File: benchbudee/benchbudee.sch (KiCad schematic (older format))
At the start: 0 parts

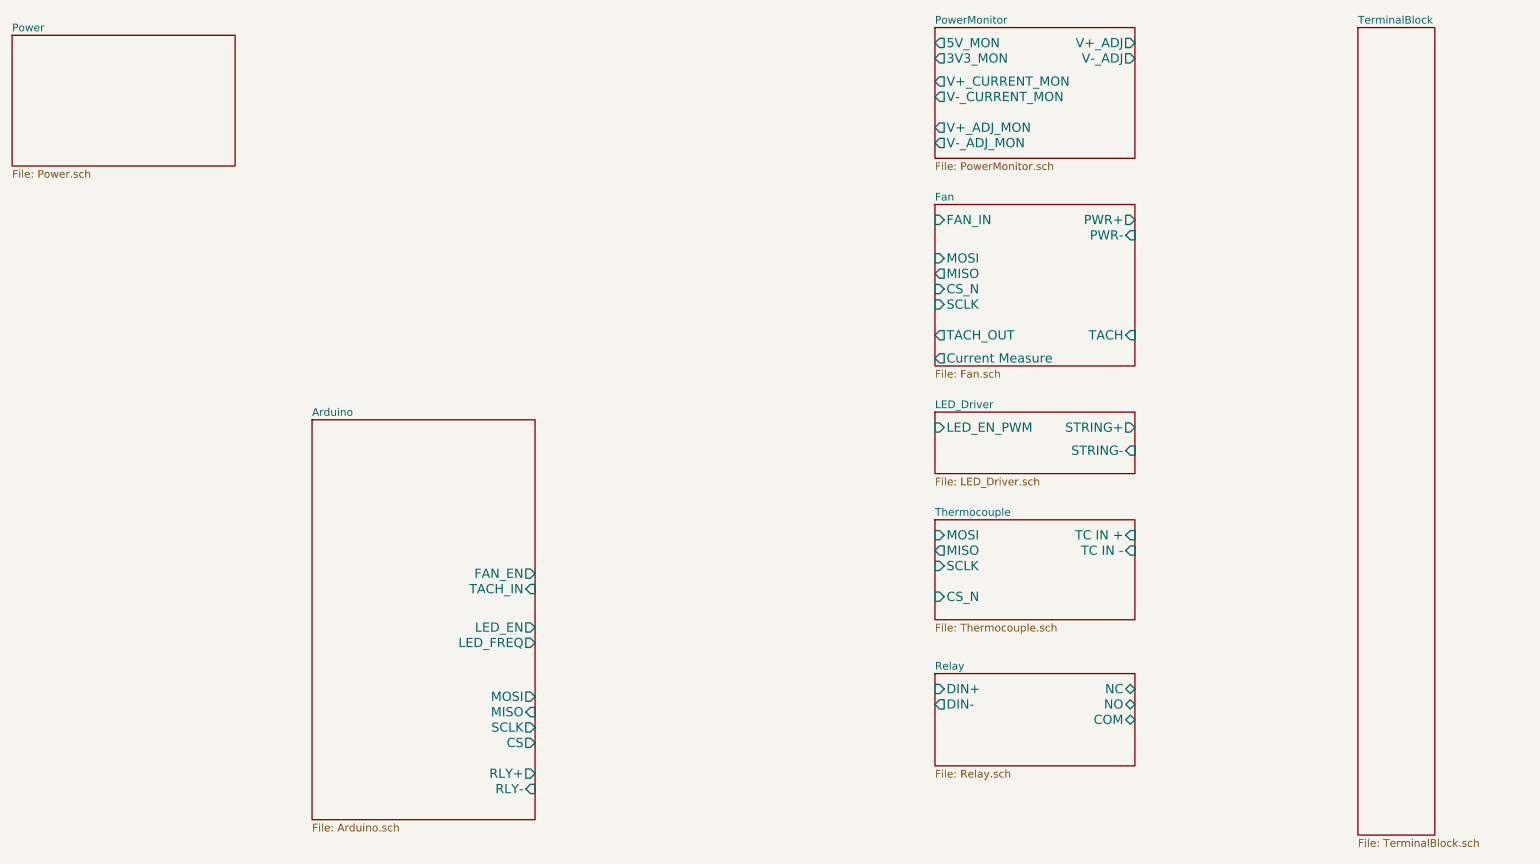
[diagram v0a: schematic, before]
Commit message: Setting up for layout
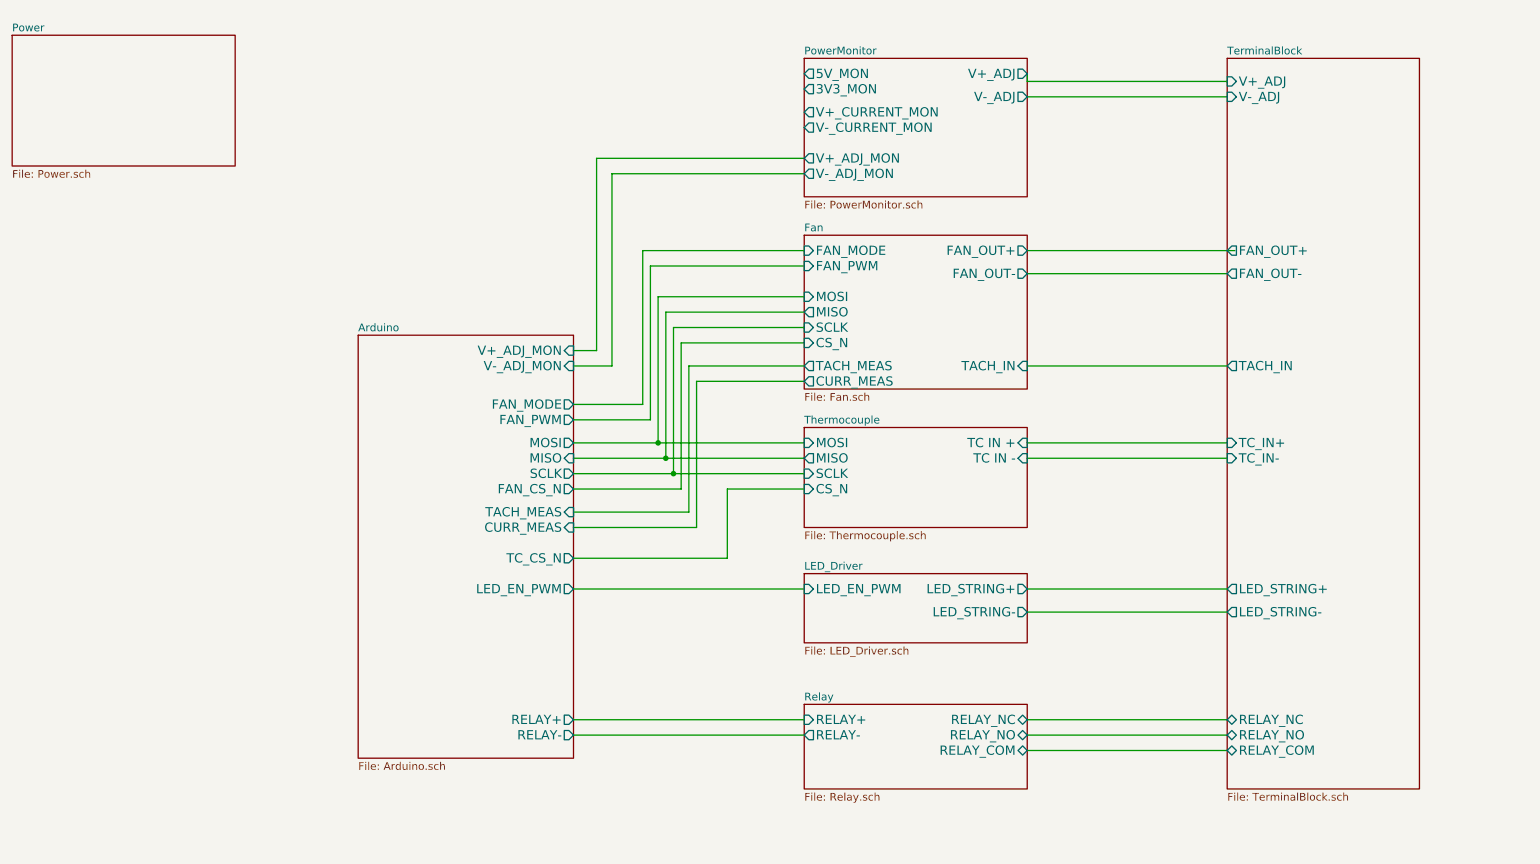
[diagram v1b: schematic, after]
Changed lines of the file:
@@
 LIBS:benchbudee-custom
 LIBS:benchbudee-cache
-EELAYER 27 0
+EELAYER 24 0
 EELAYER END
 $Descr A4 11693 8268
@@
 $EndDescr
 $Sheet
-S 3050 3450 1450 2600
-U 52F13E2E
-F0 "Arduino" 50
-F1 "Arduino.sch" 50
-F2 "RLY+" O R 4500 5750 60
-F3 "RLY-" I R 4500 5850 60
-F4 "MOSI" O R 4500 5250 60
-F5 "MISO" I R 4500 5350 60
-F6 "SCLK" O R 4500 5450 60
-F7 "CS" O R 4500 5550 60
-F8 "LED_EN" O R 4500 4800 60
-F9 "LED_FREQ" O R 4500 4900 60
-F10 "FAN_EN" O R 4500 4450 60
-F11 "TACH_IN" I R 4500 4550 60
-$EndSheet
-$Sheet
-S 7100 4100 1300 650
+S 6250 3500 1450 650
 U 52F13E8B
 F0 "Thermocouple" 50
 F1 "Thermocouple.sch" 50
-F2 "TC IN +" I R 8400 4200 60
-F3 "TC IN -" I R 8400 4300 60
-F4 "MOSI" I L 7100 4200 60
-F5 "MISO" O L 7100 4300 60
-F6 "SCLK" I L 7100 4400 60
-F7 "CS_N" I L 7100 4600 60
-$EndSheet
-$Sheet
-S 7100 5100 1300 600
+F2 "TC IN +" I R 7700 3600 60
+F3 "TC IN -" I R 7700 3700 60
+F4 "MOSI" I L 6250 3600 60
+F5 "MISO" O L 6250 3700 60
+F6 "SCLK" I L 6250 3800 60
+F7 "CS_N" I L 6250 3900 60
+$EndSheet
+$Sheet
+S 6250 5300 1450 550
 U 52F13E9E
 F0 "Relay" 50
 F1 "Relay.sch" 50
-F2 "DIN+" I L 7100 5200 60
-F3 "DIN-" O L 7100 5300 60
-F4 "NC" B R 8400 5200 60
-F5 "NO" B R 8400 5300 60
-F6 "COM" B R 8400 5400 60
+F2 "RELAY_NC" B R 7700 5400 60
+F3 "RELAY_NO" B R 7700 5500 60
+F4 "RELAY_COM" B R 7700 5600 60
+F5 "RELAY+" I L 6250 5400 60
+F6 "RELAY-" O L 6250 5500 60
 $EndSheet
 $Sheet
@@
 $EndSheet
 $Sheet
-S 7100 3400 1300 400
+S 6250 4450 1450 450
 U 52F1408A
 F0 "LED_Driver" 50
 F1 "LED_Driver.sch" 50
-F2 "STRING+" O R 8400 3500 60
-F3 "STRING-" I R 8400 3650 60
-F4 "LED_EN_PWM" I L 7100 3500 60
-$EndSheet
-$Sheet
-S 9850 900  500  5250
+F2 "LED_EN_PWM" I L 6250 4550 60
+F3 "LED_STRING+" O R 7700 4550 60
+F4 "LED_STRING-" O R 7700 4700 60
+$EndSheet
+$Sheet
+S 6250 1100 1450 900
+U 52FC1BE1
+F0 "PowerMonitor" 50
+F1 "PowerMonitor.sch" 50
+F2 "V+_ADJ" O R 7700 1200 60
+F3 "V-_ADJ" O R 7700 1350 60
+F4 "3V3_MON" O L 6250 1300 60
+F5 "5V_MON" O L 6250 1200 60
+F6 "V+_ADJ_MON" O L 6250 1750 60
+F7 "V-_ADJ_MON" O L 6250 1850 60
+F8 "V+_CURRENT_MON" O L 6250 1450 60
+F9 "V-_CURRENT_MON" O L 6250 1550 60
+$EndSheet
+Wire Wire Line
+	7700 1200 7700 1250
+Wire Wire Line
+	7700 1250 9000 1250
+Wire Wire Line
+	7700 1350 9000 1350
+Wire Wire Line
+	7700 2350 9050 2350
+Wire Wire Line
+	7700 2500 9000 2500
+Wire Wire Line
+	7700 3100 9000 3100
+Wire Wire Line
+	7700 5400 9000 5400
+Wire Wire Line
+	7700 5500 9000 5500
+Wire Wire Line
+	7700 5600 9000 5600
+Wire Wire Line
+	4750 3000 4900 3000
+Wire Wire Line
+	4900 3000 4900 1750
+Wire Wire Line
+	4900 1750 6250 1750
+Wire Wire Line
+	4750 3100 5000 3100
+Wire Wire Line
+	5000 3100 5000 1850
+Wire Wire Line
+	5000 1850 6250 1850
+Wire Wire Line
+	4750 3450 5250 3450
+Wire Wire Line
+	5250 3450 5250 2450
+Wire Wire Line
+	5250 2450 6250 2450
+Wire Wire Line
+	4750 3600 5300 3600
+Wire Wire Line
+	5300 3600 6250 3600
+Wire Wire Line
+	5300 3600 5300 2650
+Wire Wire Line
+	5300 2650 6250 2650
+Wire Wire Line
+	4750 3700 5350 3700
+Wire Wire Line
+	5350 3700 6250 3700
+Wire Wire Line
+	5350 3700 5350 2750
+Wire Wire Line
+	5350 2750 6250 2750
+Wire Wire Line
+	5400 3800 5400 2850
+Wire Wire Line
+	5400 2850 6250 2850
+Wire Wire Line
+	4750 4050 5500 4050
+Wire Wire Line
+	5500 4050 5500 3100
+Wire Wire Line
+	5500 3100 6250 3100
+Wire Wire Line
+	4750 4150 5550 4150
+Wire Wire Line
+	5550 4150 5550 3200
+Wire Wire Line
+	5550 3200 6250 3200
+Wire Wire Line
+	4750 4550 6250 4550
+$Sheet
+S 9000 1100 1250 4750
 U 52F140D2
 F0 "TerminalBlock" 50
 F1 "TerminalBlock.sch" 50
-$EndSheet
-$Sheet
-S 7100 2050 1300 1050
+F2 "V+_ADJ" I L 9000 1250 60
+F3 "V-_ADJ" I L 9000 1350 60
+F4 "FAN_OUT+" O L 9000 2350 60
+F5 "FAN_OUT-" O L 9000 2500 60
+F6 "TACH_IN" O L 9000 3100 60
+F7 "LED_STRING+" O L 9000 4550 60
+F8 "LED_STRING-" O L 9000 4700 60
+F9 "TC_IN+" I L 9000 3600 60
+F10 "TC_IN-" I L 9000 3700 60
+F11 "RELAY_NO" B L 9000 5500 60
+F12 "RELAY_NC" B L 9000 5400 60
+F13 "RELAY_COM" B L 9000 5600 60
+$EndSheet
+Wire Wire Line
+	7700 3600 9000 3600
+Wire Wire Line
+	7700 3700 9000 3700
+Wire Wire Line
+	7700 4550 9000 4550
+Wire Wire Line
+	7700 4700 9000 4700
+Connection ~ 5300 3600
+Connection ~ 5350 3700
+Wire Wire Line
+	4750 3800 5400 3800
+Wire Wire Line
+	5400 3800 6250 3800
+Connection ~ 5400 3800
+Wire Wire Line
+	4750 3900 5450 3900
+Wire Wire Line
+	5450 3900 5450 2950
+Wire Wire Line
+	5450 2950 6250 2950
+Wire Wire Line
+	4750 4350 5750 4350
+Wire Wire Line
+	5750 4350 5750 3900
+Wire Wire Line
+	5750 3900 6250 3900
+Wire Wire Line
+	4750 5400 6250 5400
+Wire Wire Line
+	6250 5500 4750 5500
+Wire Wire Line
+	4750 3350 5200 3350
+Wire Wire Line
+	5200 3350 5200 2350
+Wire Wire Line
+	5200 2350 6250 2350
+$Sheet
+S 6250 2250 1450 1000
 U 52F140AA
 F0 "Fan" 50
 F1 "Fan.sch" 50
-F2 "PWR+" O R 8400 2150 60
-F3 "PWR-" I R 8400 2250 60
-F4 "TACH" I R 8400 2900 60
-F5 "TACH_OUT" O L 7100 2900 60
-F6 "FAN_IN" I L 7100 2150 60
-F7 "Current Measure" O L 7100 3050 60
-F8 "MOSI" I L 7100 2400 60
-F9 "MISO" O L 7100 2500 60
-F10 "CS_N" I L 7100 2600 60
-F11 "SCLK" I L 7100 2700 60
-$EndSheet
-$Sheet
-S 7100 900  1300 850
-U 52FC1BE1
-F0 "PowerMonitor" 50
-F1 "PowerMonitor.sch" 50
-F2 "V+_ADJ" O R 8400 1000 60
-F3 "V-_ADJ" O R 8400 1100 60
-F4 "3V3_MON" O L 7100 1100 60
-F5 "5V_MON" O L 7100 1000 60
-F6 "V+_ADJ_MON" O L 7100 1550 60
-F7 "V-_ADJ_MON" O L 7100 1650 60
-F8 "V+_CURRENT_MON" O L 7100 1250 60
-F9 "V-_CURRENT_MON" O L 7100 1350 60
+F2 "MOSI" I L 6250 2650 60
+F3 "MISO" O L 6250 2750 60
+F4 "CS_N" I L 6250 2950 60
+F5 "SCLK" I L 6250 2850 60
+F6 "FAN_OUT+" O R 7700 2350 60
+F7 "FAN_OUT-" O R 7700 2500 60
+F8 "TACH_IN" I R 7700 3100 60
+F9 "TACH_MEAS" O L 6250 3100 60
+F10 "CURR_MEAS" O L 6250 3200 60
+F11 "FAN_PWM" I L 6250 2450 60
+F12 "FAN_MODE" I L 6250 2350 60
+$EndSheet
+$Sheet
+S 3350 2900 1400 2750
+U 52F13E2E
+F0 "Arduino" 50
+F1 "Arduino.sch" 50
+F2 "MOSI" O R 4750 3600 60
+F3 "MISO" I R 4750 3700 60
+F4 "SCLK" O R 4750 3800 60
+F5 "RELAY-" O R 4750 5500 60
+F6 "RELAY+" O R 4750 5400 60
+F7 "TACH_MEAS" I R 4750 4050 60
+F8 "CURR_MEAS" I R 4750 4150 60
+F9 "V+_ADJ_MON" I R 4750 3000 60
+F10 "V-_ADJ_MON" I R 4750 3100 60
+F11 "LED_EN_PWM" O R 4750 4550 60
+F12 "FAN_CS_N" O R 4750 3900 60
+F13 "TC_CS_N" O R 4750 4350 60
+F14 "FAN_PWM" O R 4750 3450 60
+F15 "FAN_MODE" O R 4750 3350 60
 $EndSheet
 $EndSCHEMATC

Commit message: Relay module footprints done
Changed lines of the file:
@@
 	5250 2450 6250 2450
 Wire Wire Line
-	4750 3600 5300 3600
-Wire Wire Line
-	5300 3600 6250 3600
+	4750 3600 6250 3600
 Wire Wire Line
 	5300 3600 5300 2650
@@
 	5300 2650 6250 2650
 Wire Wire Line
-	4750 3700 5350 3700
-Wire Wire Line
-	5350 3700 6250 3700
+	4750 3700 6250 3700
 Wire Wire Line
 	5350 3700 5350 2750
@@
 Connection ~ 5350 3700
 Wire Wire Line
-	4750 3800 5400 3800
-Wire Wire Line
-	5400 3800 6250 3800
+	4750 3800 6250 3800
 Connection ~ 5400 3800
 Wire Wire Line
